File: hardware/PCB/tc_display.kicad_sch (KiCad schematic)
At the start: 35 parts, among them Q1 2N2222, Q2 2N2222, U12 SA15-11SRWA, U13 SA15-11SRWA, U14 SA15-11SRWA, U15 SA15-11SRWA, U16 MAX7219, U17 SA15-11SRWA, U18 SA15-11SRWA, U19 SA15-11SRWA, U20 SA15-11SRWA, U34 SN74LV1T34DBV, U35 SN74LV1T34DBV, U36 SN74LV1T34DBV

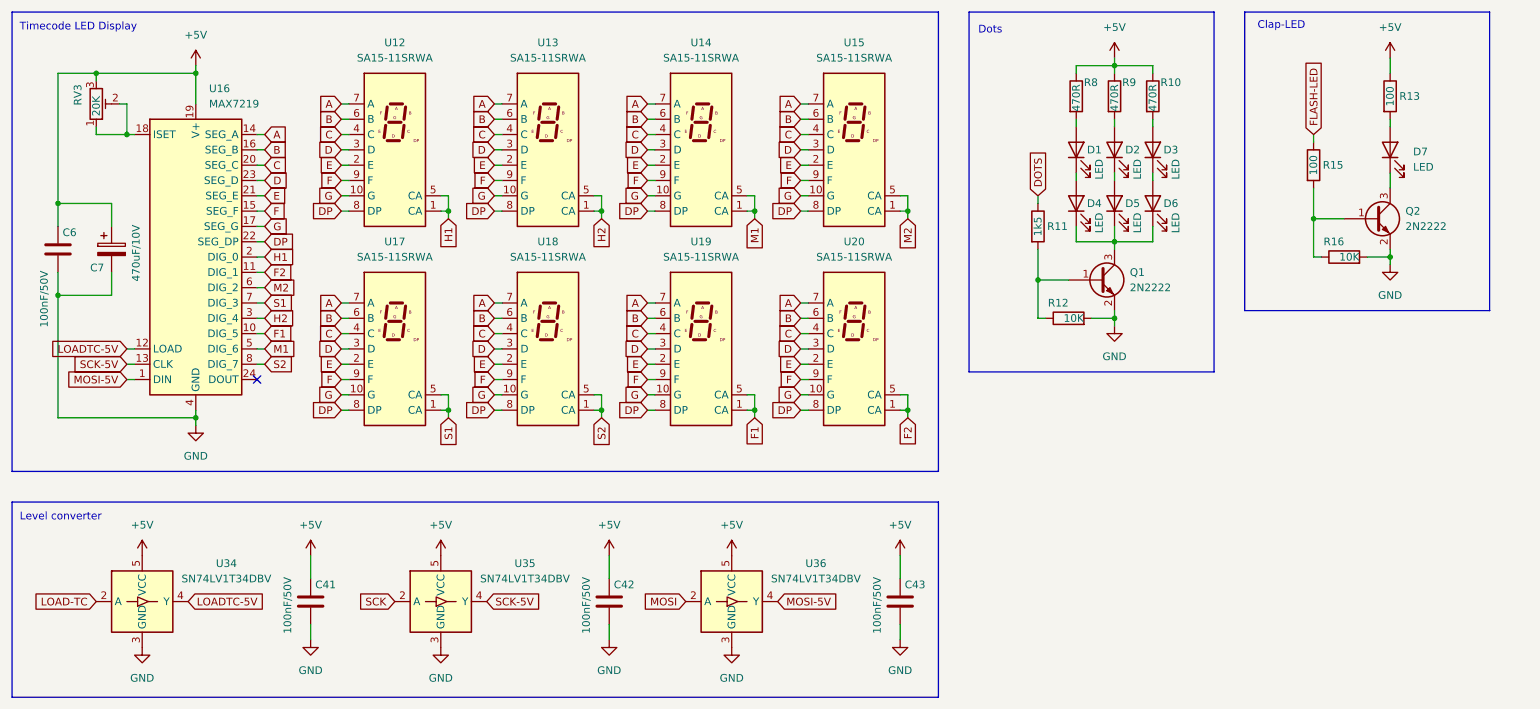
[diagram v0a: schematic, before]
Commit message: minor fixes on pcb
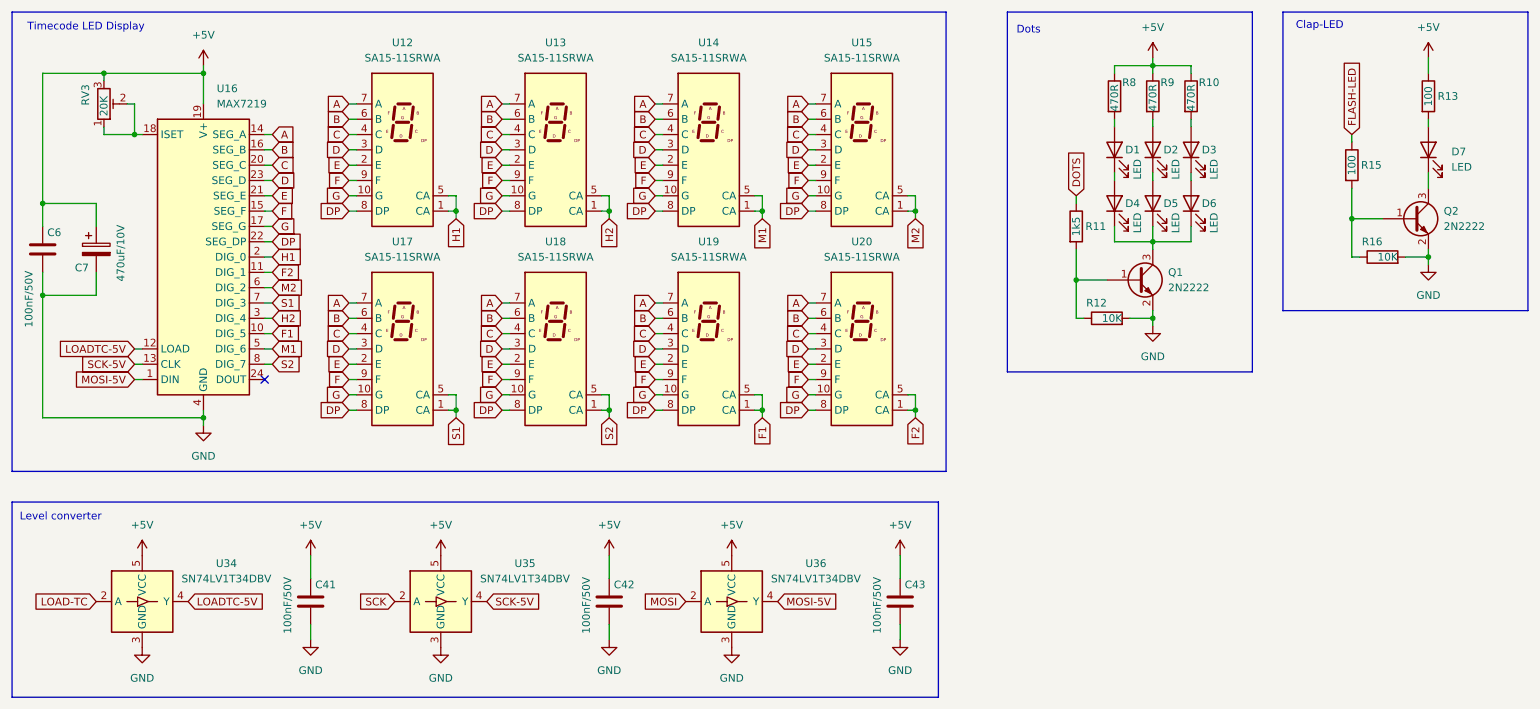
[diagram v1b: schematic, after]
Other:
- moved on the sheet: C6, C7, D1, D2, D3, D4, D5, D6, D7, Q1, Q2, R10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
